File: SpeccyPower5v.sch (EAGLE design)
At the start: 70 parts, among them T1 TRANS_ER29

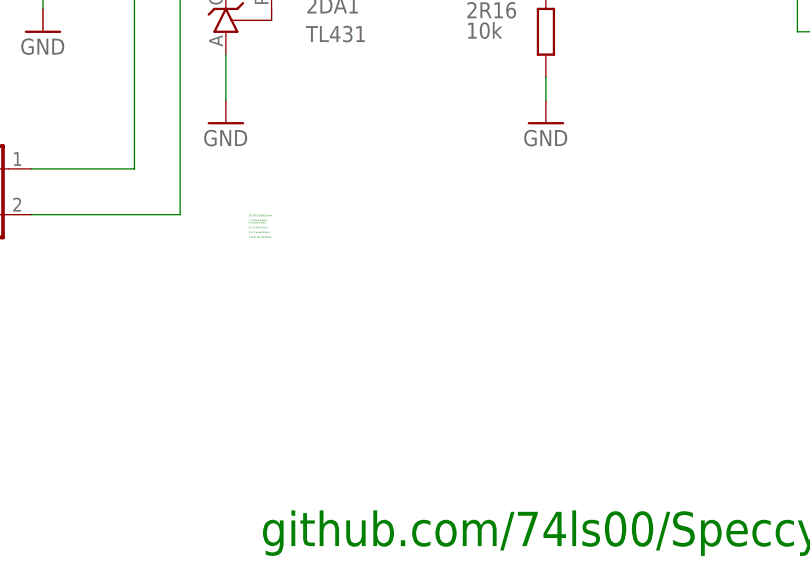
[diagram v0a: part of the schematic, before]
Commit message: ..
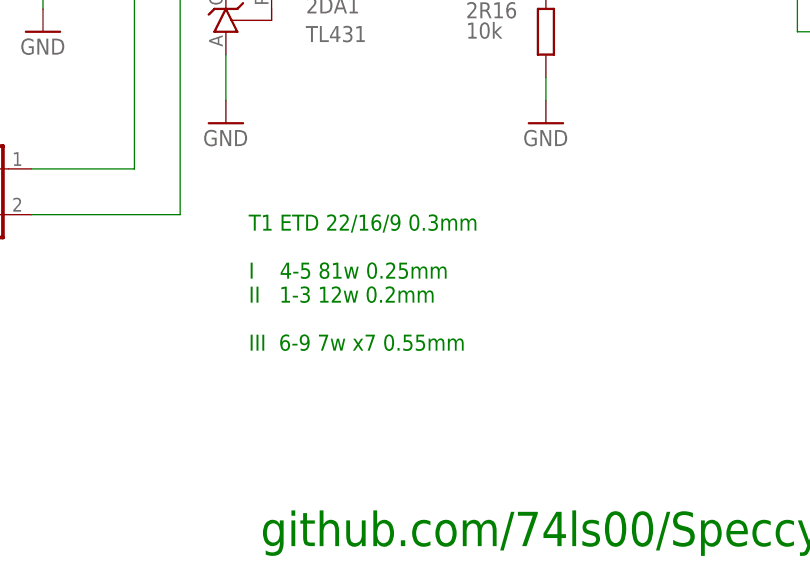
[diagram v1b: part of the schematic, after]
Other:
- note added: "T1 ETD 22/16/9 0.3mm I 4-5 81w 0.25mm II 1-3 12w 0.2mm III 6-9 7w x7 0.55mm"
- note removed: "2T1 ETD 29/16/10 2mm I 2-4 51w 0.4mm II 4-5 51w 0.4mm III 1-3 17w 0.2mm IV 6-7 5w 6x0.55mm V 10-11 8w 4x0.55mm"
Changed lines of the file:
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@@
 <plain>
 <text x="284.48" y="10.16" size="3.81" layer="91" rot="R180">github.com/74ls00/SpeccyPower5v</text>
-<text x="200.66" y="43.18" size="0.1778" layer="91" font="vector" rot="MR180">2T1 ETD 29/16/10 2mm
-I   2-4 51w 0.4mm
-II 4-5 51w 0.4mm
-III  1-3 17w 0.2mm
-IV 6-7 5w 6x0.55mm
-V 10-11 8w 4x0.55mm</text>
+<text x="200.66" y="43.18" size="1.778" layer="91" font="vector" rot="MR180">T1 ETD 22/16/9 0.3mm
+I    4-5 81w 0.25mm
+II   1-3 12w 0.2mm
+III  6-9 7w x7 0.55mm
+</text>
 <wire x1="167.64" y1="116.84" x2="167.64" y2="0" width="0.3048" layer="98" style="shortdash"/>
 <wire x1="292.1" y1="116.84" x2="167.64" y2="116.84" width="0.4064" layer="98" style="shortdash"/>
